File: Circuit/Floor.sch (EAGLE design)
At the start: 16 parts, among them M1 MOTOR, M2 MOTOR, U1 AMS1117-3.3, X2 ESP-12

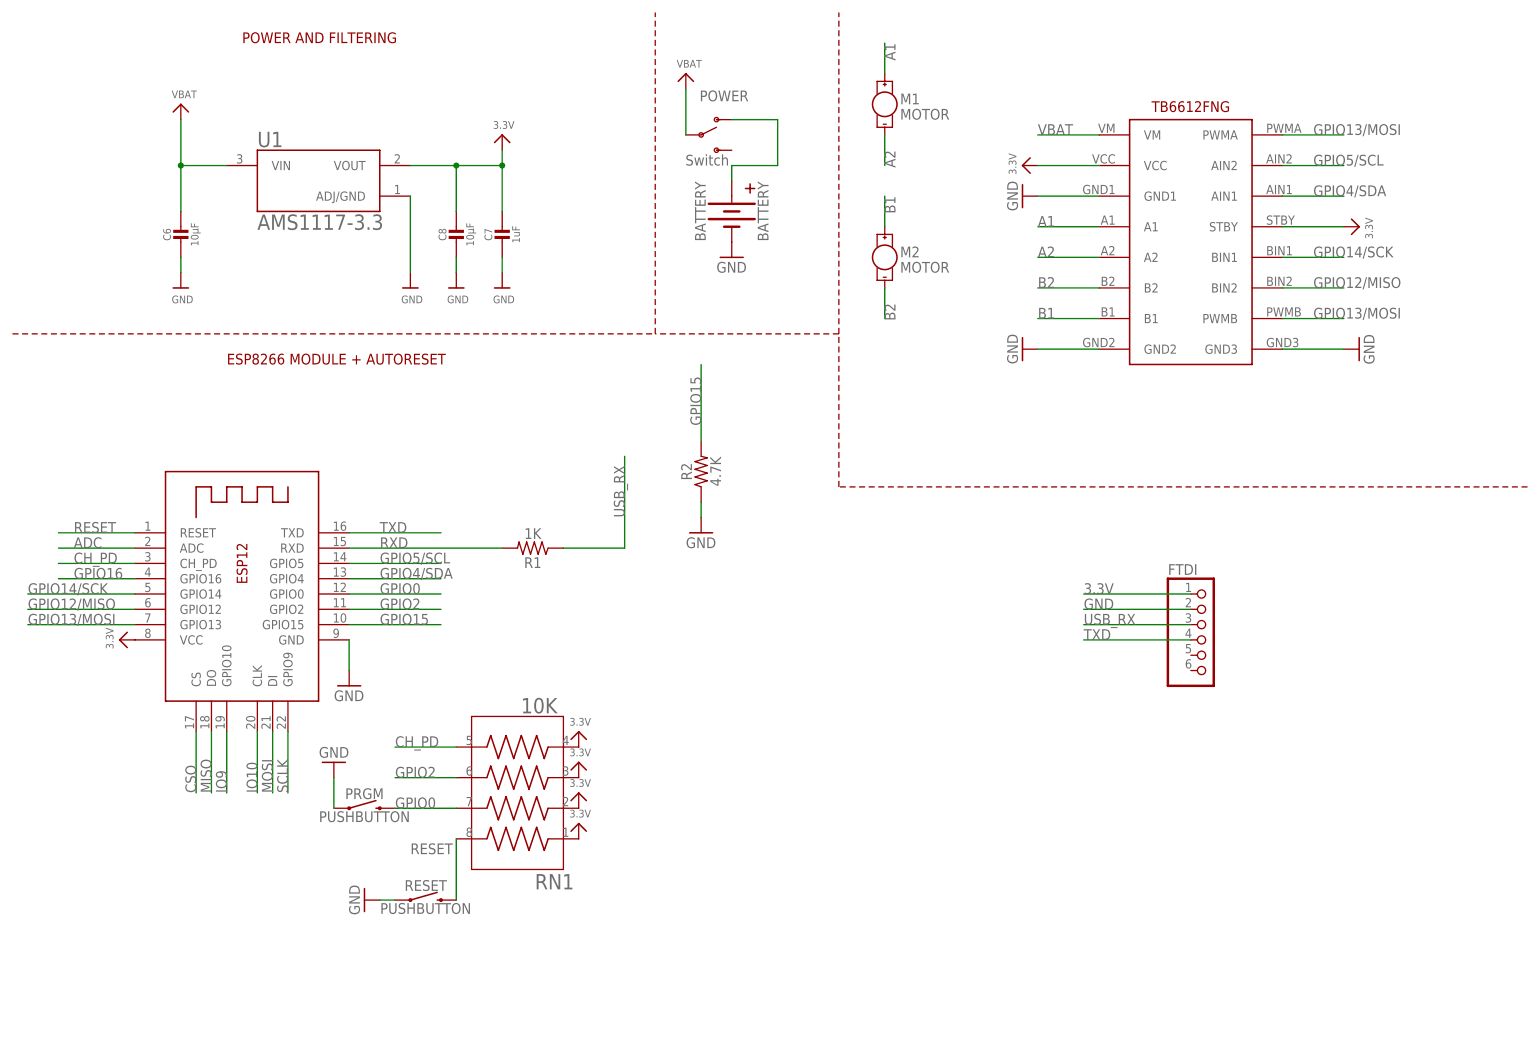
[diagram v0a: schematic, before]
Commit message: floor pcb v0
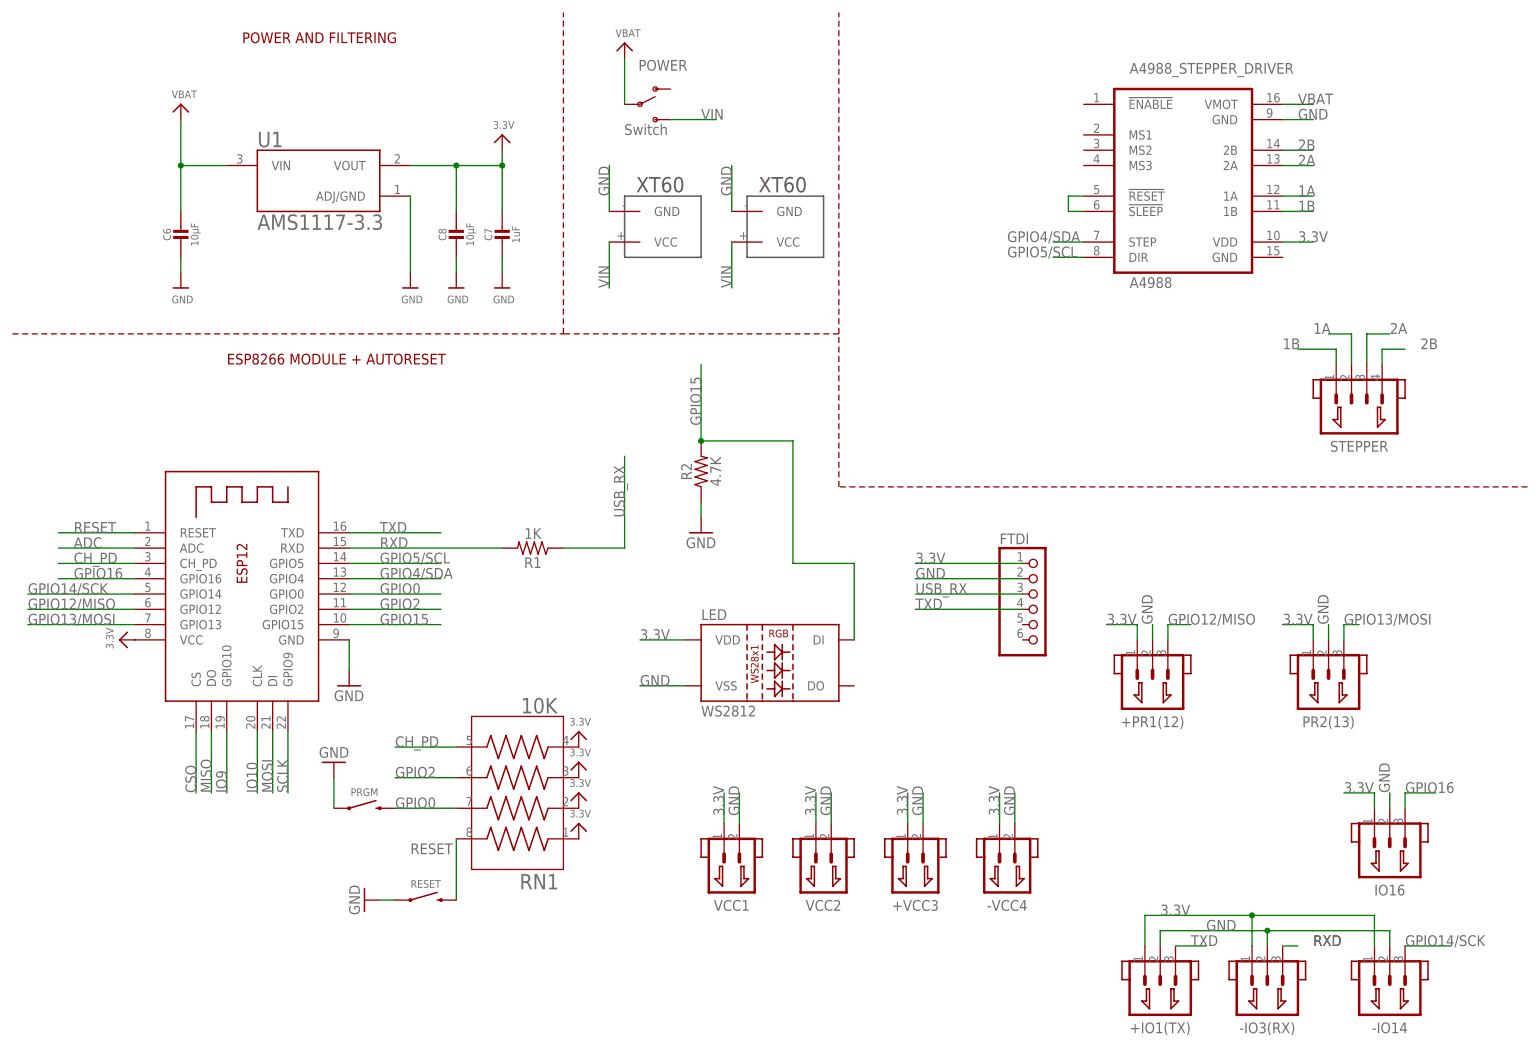
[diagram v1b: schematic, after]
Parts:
- removed BATTERY: BATTERY, AutoPark:BATTERY
- removed M1, M2: MOTOR, AutoPark:MOTOR
- removed TB1: TB6612FNG, AutoPark:TB6612FNG
- added +IO1(TX), +PR1(12), -IO14, -IO3(RX), IO16, PR2(13): XH_2.54_3P, AutoPark:XH_2.54_3P
- added +VCC3, -VCC4, VCC1, VCC2: XH_2.54_2P, AutoPark:XH_2.54_2P
- added A4988: A4988_STEPPER_DRIVER, AutoPark:A4988_STEPPER_DRIVER
- added LED: WS2812, AutoPark:WS2812
- added STEPPER: XH_2.54_4P, AutoPark:XH_2.54_4P
- added U$7, U$9: XT60, AutoPark:XT60
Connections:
- removed net A1: M1.+, TB1.A1
- removed net A2: M1.-, TB1.A2
- removed net B1: M2.+, TB1.B1
- removed net B2: M2.-, TB1.B2
- new net 1A: A4988.1A, STEPPER.2
- new net 1B: A4988.1B, STEPPER.1
- new net 2A: A4988.2A, STEPPER.3
- new net 2B: A4988.2B, STEPPER.4
- new net VIN: POWER.S, U$7.VCC, U$9.VCC
- net 3.3V: now also +IO1(TX).1, +PR1(12).1, +VCC3.1, -IO14.1, -IO3(RX).1, -VCC4.1, A4988.VDD, IO16.1, LED.VDD, PR2(13).1, VCC1.1, VCC2.1; no longer TB1.STBY, TB1.VCC
- net GND: now also +IO1(TX).2, +PR1(12).2, +VCC3.2, -IO14.2, -IO3(RX).2, -VCC4.2, A4988.GND@0, IO16.2, LED.VSS, PR2(13).2, U$7.GND, U$9.GND, VCC1.2, VCC2.2; no longer BATTERY.-, TB1.GND1, TB1.GND2, TB1.GND3
- net GPIO12/MISO: now also +PR1(12).3; no longer TB1.BIN2
- net GPIO13/MOSI: now also PR2(13).3; no longer TB1.PWMA, TB1.PWMB
- net GPIO14/SCK: now also -IO14.3; no longer TB1.BIN1
- net GPIO15: now also LED.DI
- net GPIO16: now also IO16.3
- net GPIO4/SDA: now also A4988.STEP; no longer TB1.AIN1
- net GPIO5/SCL: now also A4988.DIR; no longer TB1.AIN2
- net N$1: now also A4988.!RESET, A4988.!SLEEP; no longer BATTERY.+, POWER.O
- net RXD: now also -IO3(RX).3
- net TXD: now also +IO1(TX).3
- net VBAT: now also A4988.VMOT; no longer TB1.VM
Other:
- moved on the sheet: FTDI, POWER

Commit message: correct flipped xh conns
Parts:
- X2: device microbuilder:ESP-12E -> AutoPark:MICROBUILDER_ESP-12E
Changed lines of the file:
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@@
 <setting verticaltext="up"/>
 </settings>
-<grid distance="0.05" unitdist="inch" unit="inch" style="lines" multiple="1" display="no" altdistance="0.01" altunitdist="inch" altunit="inch"/>
+<grid distance="0.1" unitdist="inch" unit="inch" style="lines" multiple="1" display="no" altdistance="0.01" altunitdist="inch" altunit="inch"/>
 <layers>
 <layer number="1" name="Top" color="4" fill="1" visible="no" active="no"/>
@@
 <part name="U$29" library="microbuilder" deviceset="GND" device=""/>
 <part name="U$30" library="microbuilder" deviceset="GND" device=""/>
-<part name="X2" library="microbuilder" deviceset="ESP-12E" device="" value="ESP-12"/>
+<part name="X2" library="AutoPark" deviceset="MICROBUILDER_ESP-12E" device="" value="ESP-12"/>
 <part name="U$2" library="microbuilder" deviceset="3.3V" device=""/>
 <part name="GND3" library="supply1" deviceset="GND" device=""/>

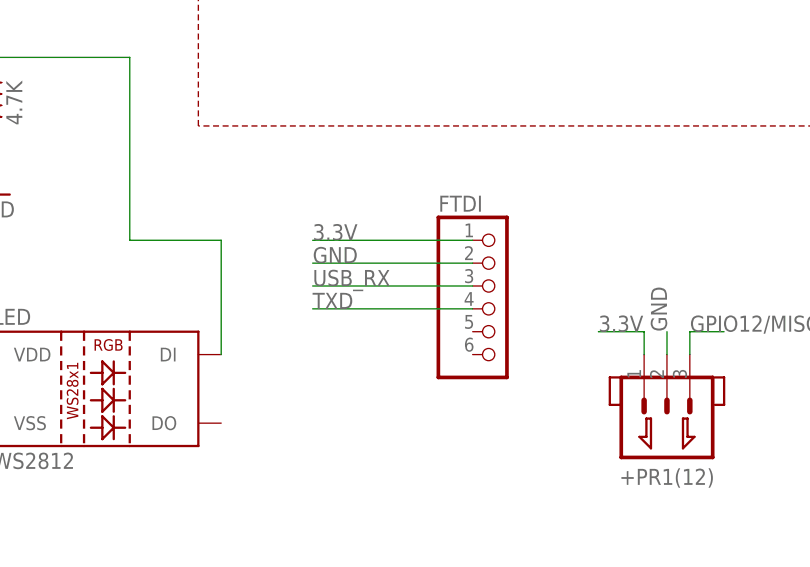
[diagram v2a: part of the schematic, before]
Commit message: floor pcb, led library, espnow wip
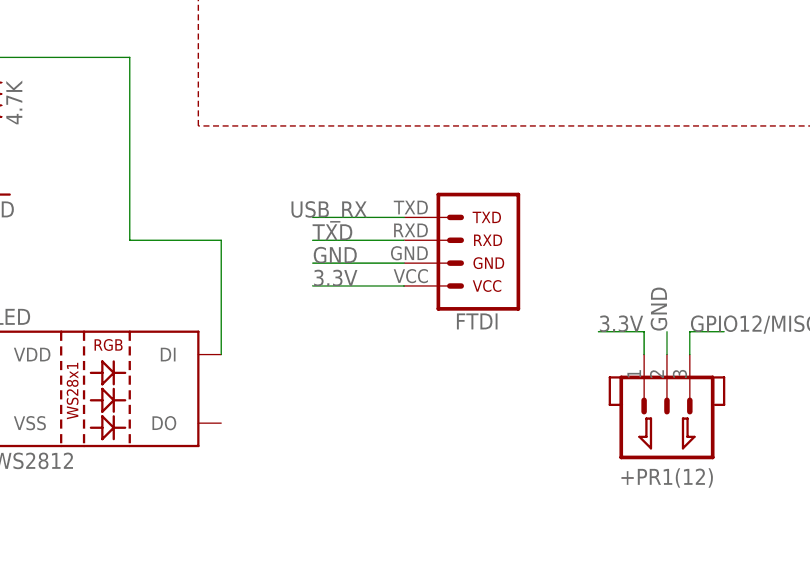
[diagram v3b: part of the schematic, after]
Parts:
- removed FTDI: (no value), pinhead:PINHD-1X6
- added U$11: FTDI, AutoPark:FTDI
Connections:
- net 3.3V: now also U$11.VCC; no longer FTDI.1
- net GND: now also U$11.GND; no longer FTDI.2
- net TXD: now also U$11.RXD; no longer FTDI.4
- net USB_RX: now also U$11.TXD; no longer FTDI.3
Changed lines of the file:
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@@
 <part name="R2" library="SparkFun-Resistors" library_urn="urn:adsk.eagle:library:532" deviceset="RESISTOR" device="1206" package3d_urn="urn:adsk.eagle:package:39654/1" value="4.7K"/>
 <part name="R1" library="SparkFun-Resistors" library_urn="urn:adsk.eagle:library:532" deviceset="RESISTOR" device="1206" package3d_urn="urn:adsk.eagle:package:39654/1" value="1K"/>
-<part name="FTDI" library="pinhead" library_urn="urn:adsk.eagle:library:325" deviceset="PINHD-1X6" device="" package3d_urn="urn:adsk.eagle:package:22472/2"/>
 <part name="U$3" library="microbuilder" deviceset="3.3V" device=""/>
 <part name="GND4" library="supply1" deviceset="GND" device=""/>
@@
 <part name="PR2(13)" library="AutoPark" deviceset="XH_2.54_3P" device=""/>
 <part name="IO16" library="AutoPark" deviceset="XH_2.54_3P" device=""/>
+<part name="U$11" library="AutoPark" deviceset="FTDI" device=""/>
 </parts>
 <sheets>
@@
 <attribute name="VALUE" x="91.44" y="87.884" size="1.778" layer="96" font="vector" rot="R180" align="top-center"/>
 </instance>
-<instance part="FTDI" gate="A" x="175.26" y="76.2">
-<attribute name="NAME" x="168.91" y="86.995" size="1.778" layer="95"/>
-<attribute name="VALUE" x="168.91" y="66.04" size="1.778" layer="96"/>
-</instance>
 <instance part="U$3" gate="G$1" x="99.06" y="45.72">
 <attribute name="VALUE" x="97.536" y="46.736" size="1.27" layer="96"/>
@@
 <attribute name="NAME" x="233.68" y="30.48" size="1.778" layer="95" font="vector" align="top-center"/>
 </instance>
+<instance part="U$11" gate="G$1" x="170.18" y="83.82" rot="R180"/>
 </instances>
 <busses>
@@
 <wire x1="68.58" y1="27.94" x2="66.04" y2="27.94" width="0.1524" layer="91"/>
 <pinref part="RESET" gate="G$1" pin="1"/>
-</segment>
-<segment>
-<pinref part="FTDI" gate="A" pin="2"/>
-<wire x1="172.72" y1="81.28" x2="154.94" y2="81.28" width="0.1524" layer="91"/>
-<label x="154.94" y="81.28" size="1.778" layer="95"/>
 </segment>
 <segment>
@@
 <wire x1="171.45" y1="40.64" x2="171.45" y2="45.72" width="0.1524" layer="91"/>
 <label x="171.45" y="41.91" size="1.778" layer="95" rot="R90"/>
+</segment>
+<segment>
+<pinref part="U$11" gate="G$1" pin="GND"/>
+<wire x1="165.1" y1="81.28" x2="154.94" y2="81.28" width="0.1524" layer="91"/>
+<label x="154.94" y="81.28" size="1.778" layer="95"/>
 </segment>
 </net>
@@
 </segment>
 <segment>
-<pinref part="FTDI" gate="A" pin="1"/>
-<wire x1="172.72" y1="83.82" x2="154.94" y2="83.82" width="0.1524" layer="91"/>
-<label x="154.94" y="83.82" size="1.778" layer="95"/>
-</segment>
-<segment>
 <pinref part="RN1" gate="G$1" pin="2"/>
 <pinref part="U$3" gate="G$1" pin="3.3V"/>
@@
 <label x="168.91" y="41.91" size="1.778" layer="95" rot="R90"/>
 </segment>
+<segment>
+<pinref part="U$11" gate="G$1" pin="VCC"/>
+<wire x1="165.1" y1="78.74" x2="154.94" y2="78.74" width="0.1524" layer="91"/>
+<label x="154.94" y="78.74" size="1.778" layer="95"/>
+</segment>
 </net>
 <net name="RESET" class="0">
@@
 </segment>
 <segment>
-<pinref part="FTDI" gate="A" pin="4"/>
-<wire x1="172.72" y1="76.2" x2="154.94" y2="76.2" width="0.1524" layer="91"/>
-<label x="154.94" y="76.2" size="1.778" layer="95"/>
-</segment>
-<segment>
 <pinref part="+IO1(TX)" gate="G$1" pin="3"/>
 <wire x1="198.12" y1="20.32" x2="203.2" y2="20.32" width="0.1524" layer="91"/>
 <label x="200.66" y="20.32" size="1.778" layer="95"/>
+</segment>
+<segment>
+<pinref part="U$11" gate="G$1" pin="RXD"/>
+<wire x1="165.1" y1="83.82" x2="154.94" y2="83.82" width="0.1524" layer="91"/>
+<label x="154.94" y="83.82" size="1.778" layer="95"/>
 </segment>
 </net>
@@
 </segment>
 <segment>
-<pinref part="FTDI" gate="A" pin="3"/>
-<wire x1="172.72" y1="78.74" x2="154.94" y2="78.74" width="0.1524" layer="91"/>
-<label x="154.94" y="78.74" size="1.778" layer="95"/>
-</segment>
-</net>
+<pinref part="U$11" gate="G$1" pin="TXD"/>
+<wire x1="165.1" y1="86.36" x2="154.94" y2="86.36" width="0.1524" layer="91"/>
+<label x="152.4" y="86.36" size="1.778" layer="95"/>
+</segment>
+</net>
